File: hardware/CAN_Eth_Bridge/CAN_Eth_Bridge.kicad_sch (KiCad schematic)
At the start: 22 parts, among them J101 Global LV and CAN, J102 Conn_01x05_Pin, SW102 SW_Push, U101 AP7384-50SA, U102 AP7381-33SA-7, U103 MCP2542FDxMF, U104 XMSM0G3507SDGS28R

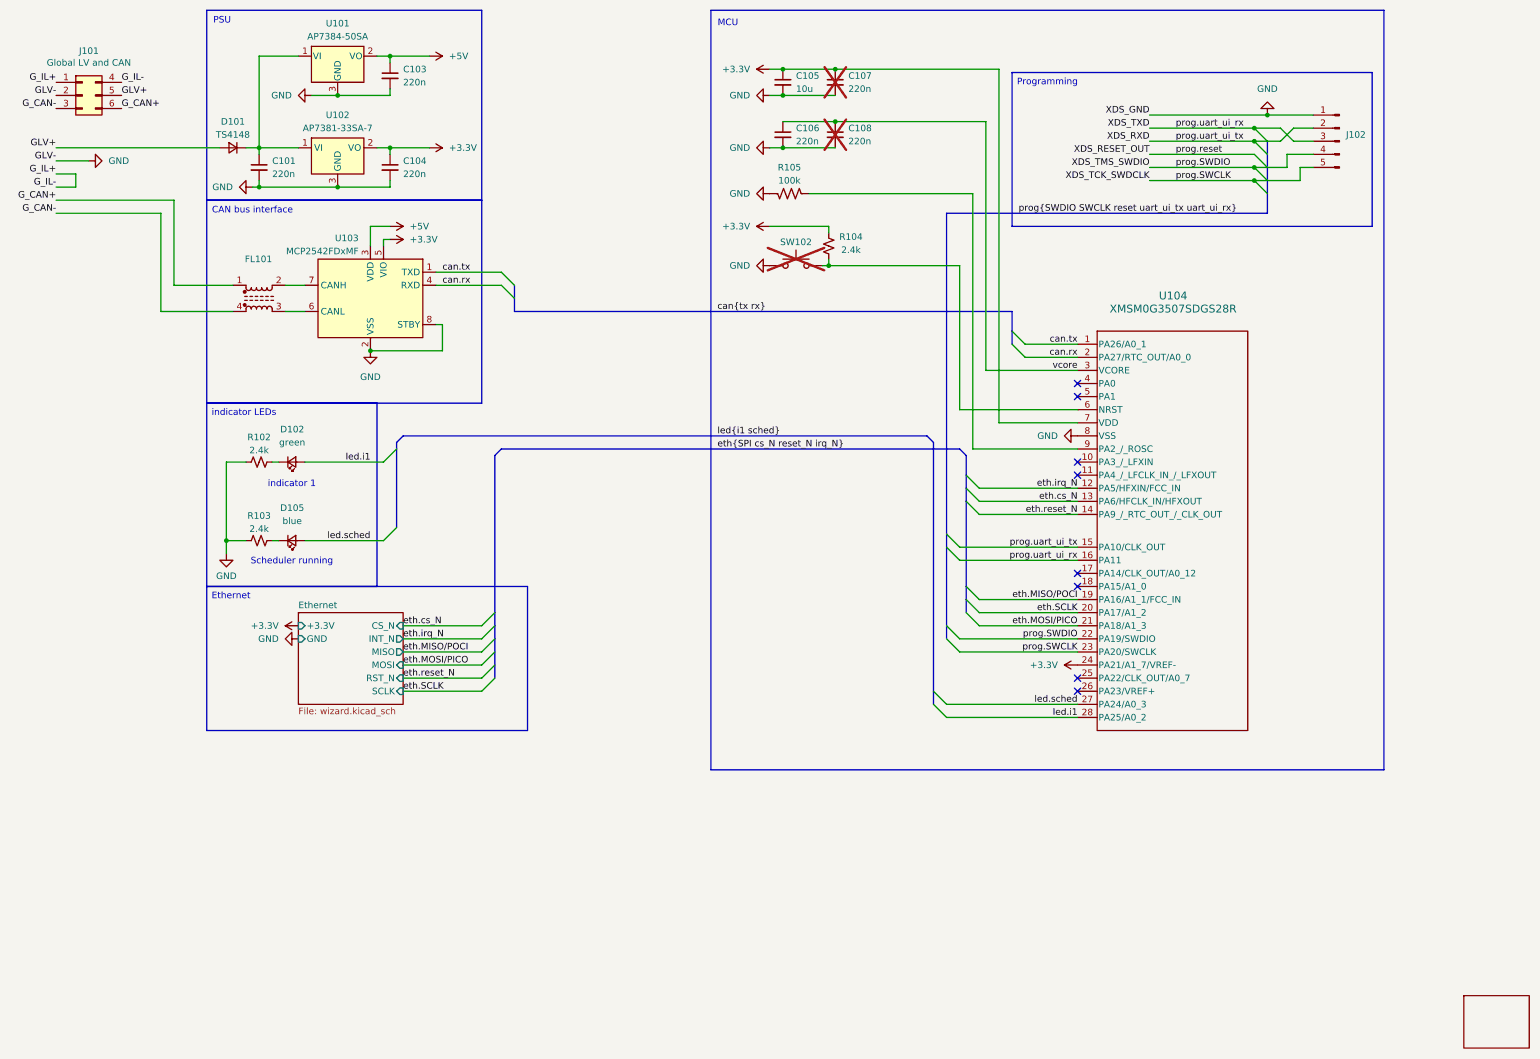
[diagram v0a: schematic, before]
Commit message: civilized note taking
and untaking !?!?!
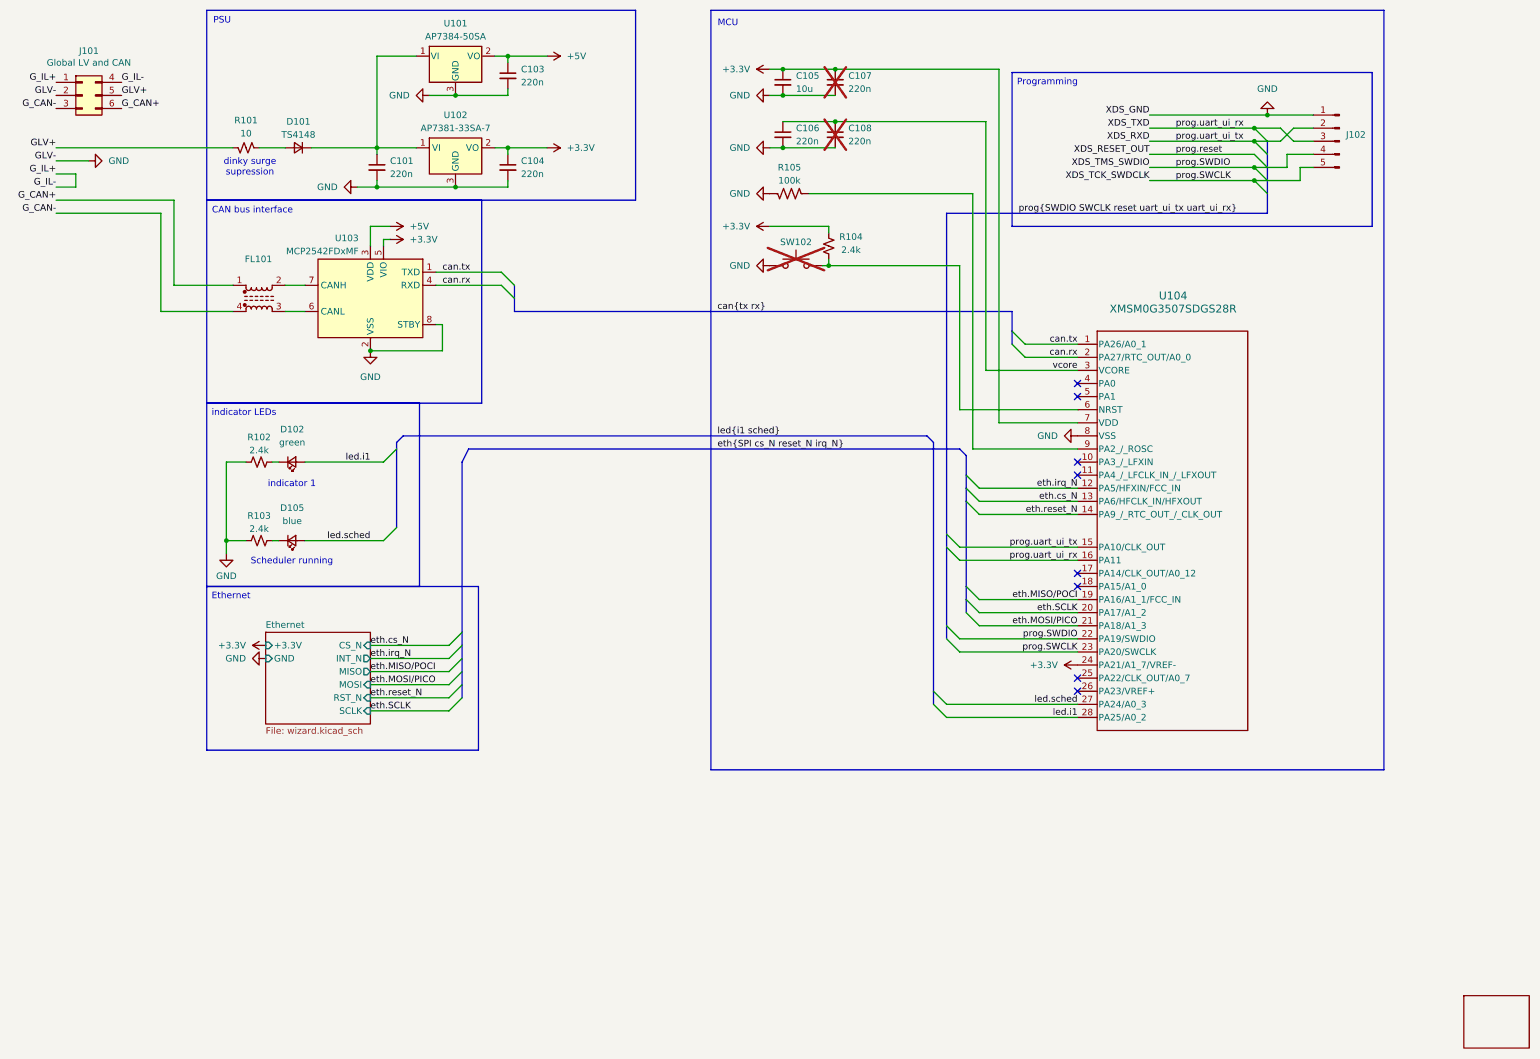
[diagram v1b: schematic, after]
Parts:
- added R101: 10, Resistor_SMD:R_0805_2012Metric_Pad1.20x1.40mm_HandSolder, symbol Device:R_Small_US
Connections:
- net GLV+: now also R101.2; no longer D101.2 (A)
- new net: D101.2 (A), R101.1
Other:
- note added: "dinky surge supression"
- moved on the sheet: C101, C103, C104, D101, U101, U102
